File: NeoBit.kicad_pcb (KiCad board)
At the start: 2 copper layers, 67.3 x 45.7 mm, 13 parts, among them J2 Barrel_Jack_MountingPin, J4 NeoPixels, J5 microbit_edge_connector, U1 74AHCT125, U2 MCP1702-3302E_TO92

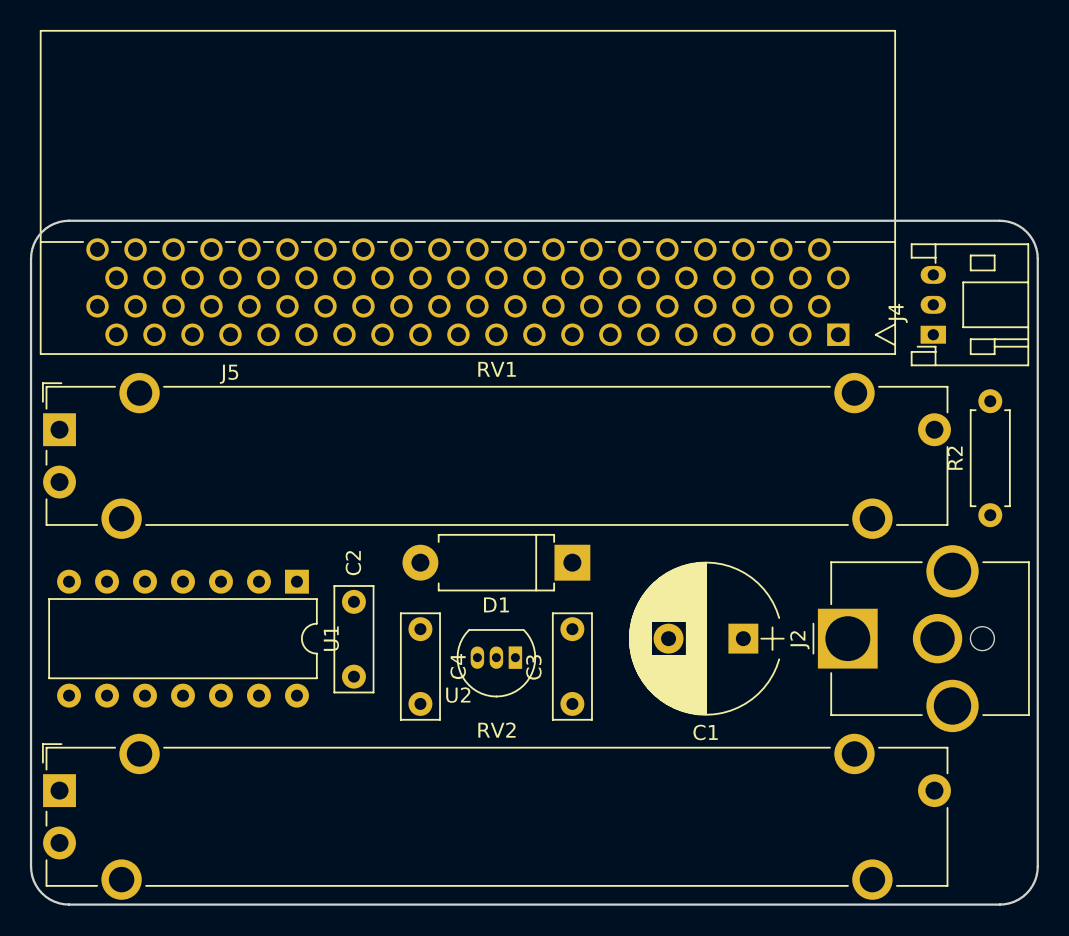
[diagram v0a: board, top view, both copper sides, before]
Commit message: Position text.
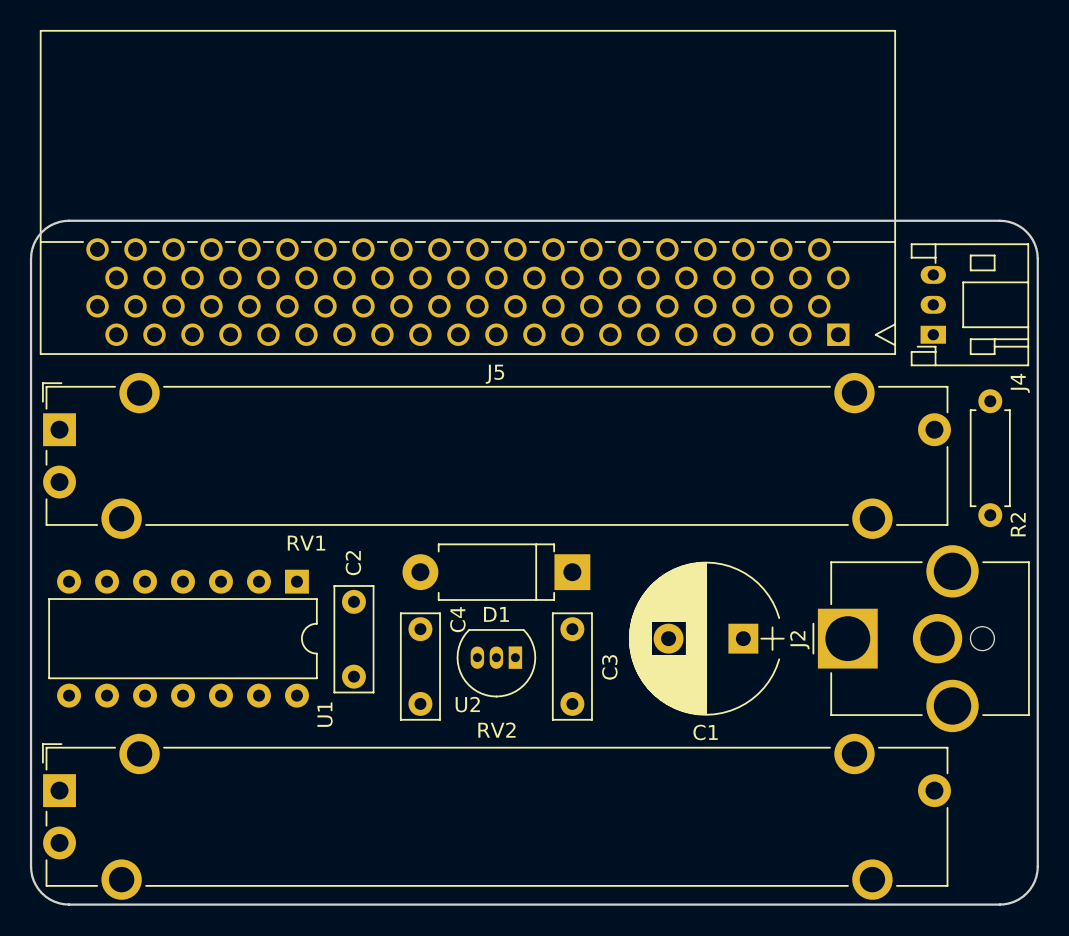
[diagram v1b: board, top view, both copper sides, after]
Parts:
- moved D1 0.63 mm to (154.9, 107.3)
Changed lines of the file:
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@@
     (descr "C, Rect series, Radial, pin pitch=5.00mm, , length*width=7*2.5mm^2, Capacitor")
     (tags "C Rect series Radial pin pitch 5.00mm  length 7mm width 2.5mm Capacitor")
-    (fp_text reference C3 (at 2.54 2.54 270) (layer F.SilkS)
+    (fp_text reference C3 (at 2.54 -2.54 270) (layer F.SilkS)
       (effects (font (size 1 1) (thickness 0.15)))
     )
@@
     (descr "C, Rect series, Radial, pin pitch=5.00mm, , length*width=7*2.5mm^2, Capacitor")
     (tags "C Rect series Radial pin pitch 5.00mm  length 7mm width 2.5mm Capacitor")
-    (fp_text reference C4 (at 2.5 -2.56 270) (layer F.SilkS)
+    (fp_text reference C4 (at -0.635 -2.54 270) (layer F.SilkS)
       (effects (font (size 1 1) (thickness 0.15)))
     )
@@
   )
   (module Diodes_THT:D_DO-15_P10.16mm_Horizontal (layer F.Cu)
-    (at 154.94 106.68 180)
+    (at 154.94 107.315 180)
     (descr "D, DO-15 series, Axial, Horizontal, pin pitch=10.16mm, , length*diameter=7.6*3.6mm^2, , http://www.diodes.com/_files/packages/DO-15.pdf")
     (tags "D DO-15 series Axial Horizontal pin pitch 10.16mm  length 7.6mm diameter 3.6mm")
@@
     (descr "JST PH series connector, S3B-PH-K, side entry type, through hole, Datasheet: http://www.jst-mfg.com/product/pdf/eng/ePH.pdf")
     (tags "connector jst ph")
-    (fp_text reference J4 (at 1.5 -2.45 90) (layer F.SilkS)
+    (fp_text reference J4 (at -3.175 5.715 90) (layer F.SilkS)
       (effects (font (size 1 1) (thickness 0.15)))
     )
@@
     (descr "Resistor, Axial_DIN0207 series, Axial, Horizontal, pin pitch=7.62mm, 0.25W = 1/4W, length*diameter=6.3*2.5mm^2, http://cdn-reichelt.de/documents/datenblatt/B400/1_4W%23YAG.pdf")
     (tags "Resistor Axial_DIN0207 series Axial Horizontal pin pitch 7.62mm 0.25W = 1/4W length 6.3mm diameter 2.5mm")
-    (fp_text reference R2 (at 3.81 -2.31 90) (layer F.SilkS)
+    (fp_text reference R2 (at -0.635 1.905 90) (layer F.SilkS)
       (effects (font (size 1 1) (thickness 0.15)))
     )
@@
     (descr "14-lead though-hole mounted DIP package, row spacing 7.62 mm (300 mils)")
     (tags "THT DIP DIL PDIP 2.54mm 7.62mm 300mil")
-    (fp_text reference U1 (at 3.81 -2.33 270) (layer F.SilkS)
+    (fp_text reference U1 (at 8.89 -1.905 270) (layer F.SilkS)
       (effects (font (size 1 1) (thickness 0.15)))
     )
@@
     (descr "TO-92 leads in-line, narrow, oval pads, drill 0.6mm (see NXP sot054_po.pdf)")
     (tags "to-92 sc-43 sc-43a sot54 PA33 transistor")
-    (fp_text reference U2 (at 3.81 -2.54 180) (layer F.SilkS)
+    (fp_text reference U2 (at 3.175 -3.175 180) (layer F.SilkS)
       (effects (font (size 1 1) (thickness 0.15)))
     )
@@
     (descr "BBC micro:bit right-angle edge connector")
     (tags "bbc microbit edge connector right-angle")
-    (fp_text reference J5 (at 40.64 -2.54 180) (layer F.SilkS)
+    (fp_text reference J5 (at 22.86 -2.54 180) (layer F.SilkS)
       (effects (font (size 1 1) (thickness 0.15)))
     )
@@
     (descr "Bourns single-gang slide potentiometer, 45mm travel")
     (tags "Bourns single-gang slide potentiometer 45mm")
-    (fp_text reference RV1 (at 29.25 -4) (layer F.SilkS)
-      (effects (font (size 1 1) (thickness 0.15)))
-    )
+    (fp_text reference RV1 (at 16.51 7.62) (layer F.SilkS)
+      (effects (font (size 1 1) (thickness 0.15)))
+    )
